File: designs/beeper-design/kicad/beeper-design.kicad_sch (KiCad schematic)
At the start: 0 parts

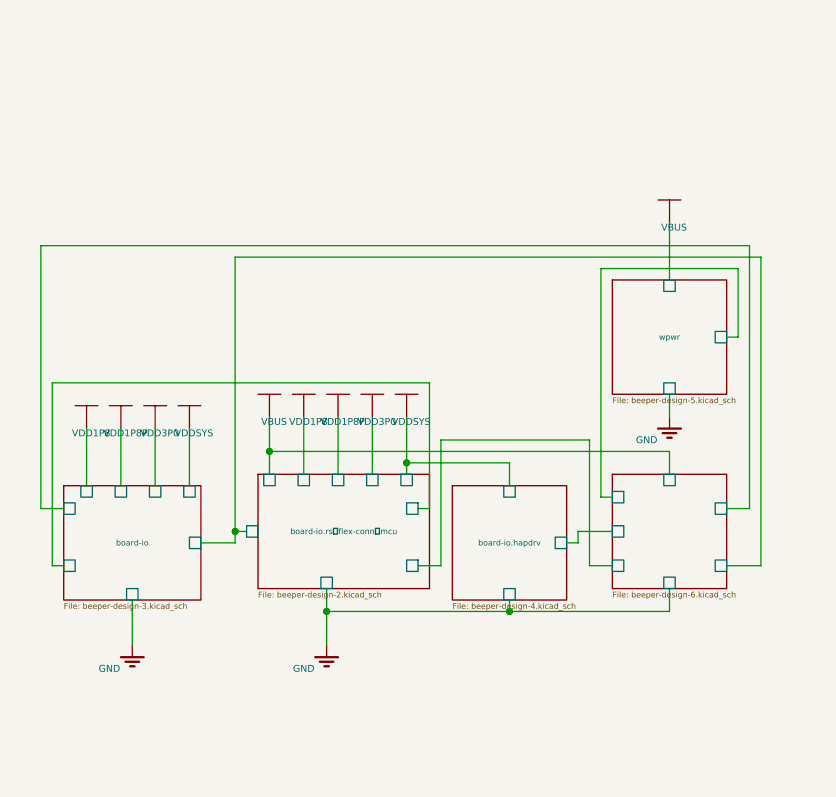
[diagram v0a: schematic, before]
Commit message: latest fully routed version
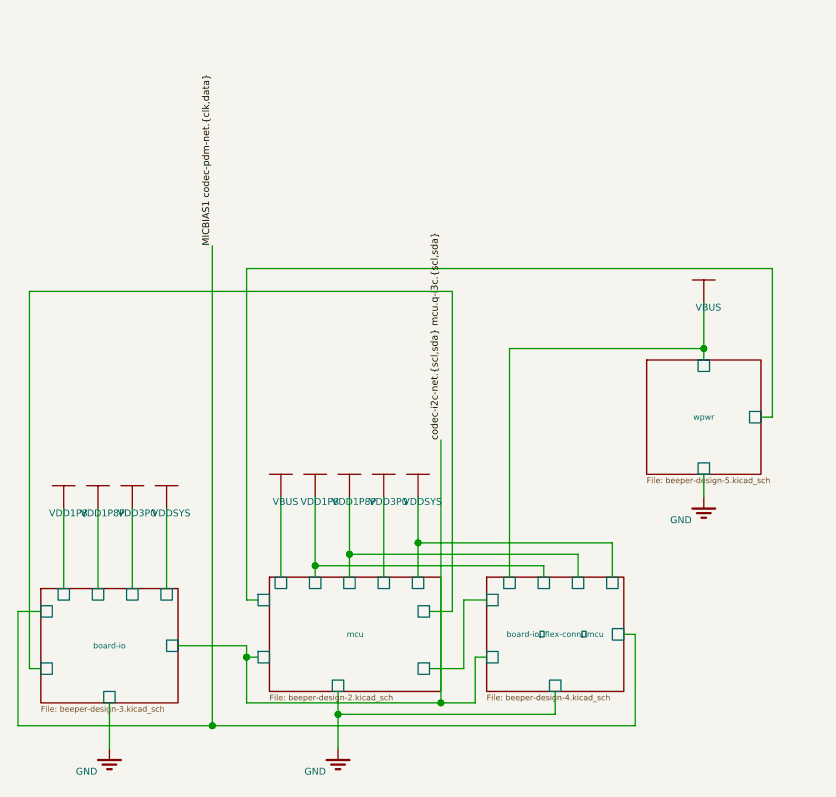
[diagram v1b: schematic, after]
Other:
- removed sheet 
- removed sheet board-io.hapdrv
- removed sheet board-io.rs flex-conn mcu
- added sheet board-io flex-conn mcu (beeper-design-4.kicad_sch)
- added sheet mcu (beeper-design-2.kicad_sch)
